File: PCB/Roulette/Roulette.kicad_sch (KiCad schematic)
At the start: 266 parts, among them J1 USB-PROG, J2 Shelly, J3 Conn_01x03, J4 Conn_01x02, Q1 PMF170XP,115, SW1 SW_Push, U2 ESP32-S3-MINI-1

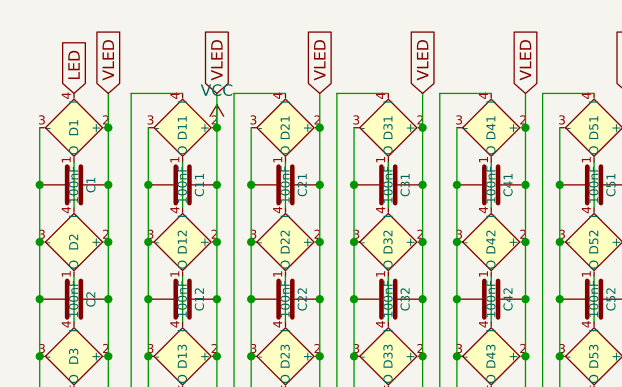
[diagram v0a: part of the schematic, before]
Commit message: Library update
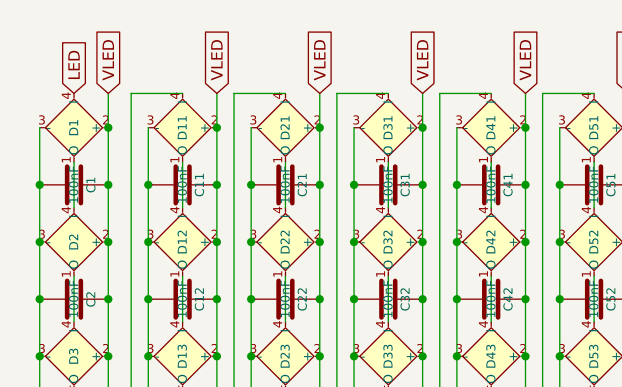
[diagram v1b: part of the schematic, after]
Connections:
- net VCC renamed VLED
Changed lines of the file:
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@@
   (junction (at 35.56 139.065) (diameter 0) (color 0 0 0 0)
   )
-  (junction (at 8.89 24.765) (diameter 0) (color 0 0 0 0)
-  )
   (junction (at 290.83 55.88) (diameter 0) (color 0 0 0 0)
   )
@@
   (junction (at 31.75 94.615) (diameter 0) (color 0 0 0 0)
   )
+  (junction (at 8.89 24.765) (diameter 0) (color 0 0 0 0)
+  )
   (junction (at 208.915 53.975) (diameter 0) (color 0 0 0 0)
   )
@@
     (stroke (width 0) (type default))
   )
-  (wire (pts (xy 8.89 20.955) (xy 8.89 24.765))
-    (stroke (width 0) (type default))
-  )
   (wire (pts (xy 58.42 31.115) (xy 58.42 37.465))
     (stroke (width 0) (type default))
@@
     (stroke (width 0) (type default))
   )
+  (wire (pts (xy 8.89 20.955) (xy 8.89 24.765))
+    (stroke (width 0) (type default))
+  )
   (wire (pts (xy 145.415 76.835) (xy 146.05 76.835))
     (stroke (width 0) (type default))
@@
         )
       )
-    )
-  )
-  (symbol (lib_id "power:VCC") (at 8.89 24.765 0) (unit 1)
-    (in_bom yes) (on_board yes) (dnp no) (fields_autoplaced)
-    (property "Reference" "#PWR03" (at 8.89 28.575 0)
-      (effects (font (size 1.27 1.27)) hide)
-    )
-    (property "Value" "VCC" (at 8.89 20.6319 0)
-      (effects (font (size 1.27 1.27)))
-    )
-    (property "Footprint" "" (at 8.89 24.765 0)
-      (effects (font (size 1.27 1.27)) hide)
-    )
-    (property "Datasheet" "" (at 8.89 24.765 0)
-      (effects (font (size 1.27 1.27)) hide)
-    )
-    (pin "1")
-    (instances
-      (project "Roulette"
-        (path "/46c350bb-7de4-4e81-aafd-4af55e37aab0"
-          (reference "#PWR03") (unit 1)
-        )
-      )
